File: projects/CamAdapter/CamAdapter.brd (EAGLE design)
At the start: 25.4 x 41.9 mm, 5 parts

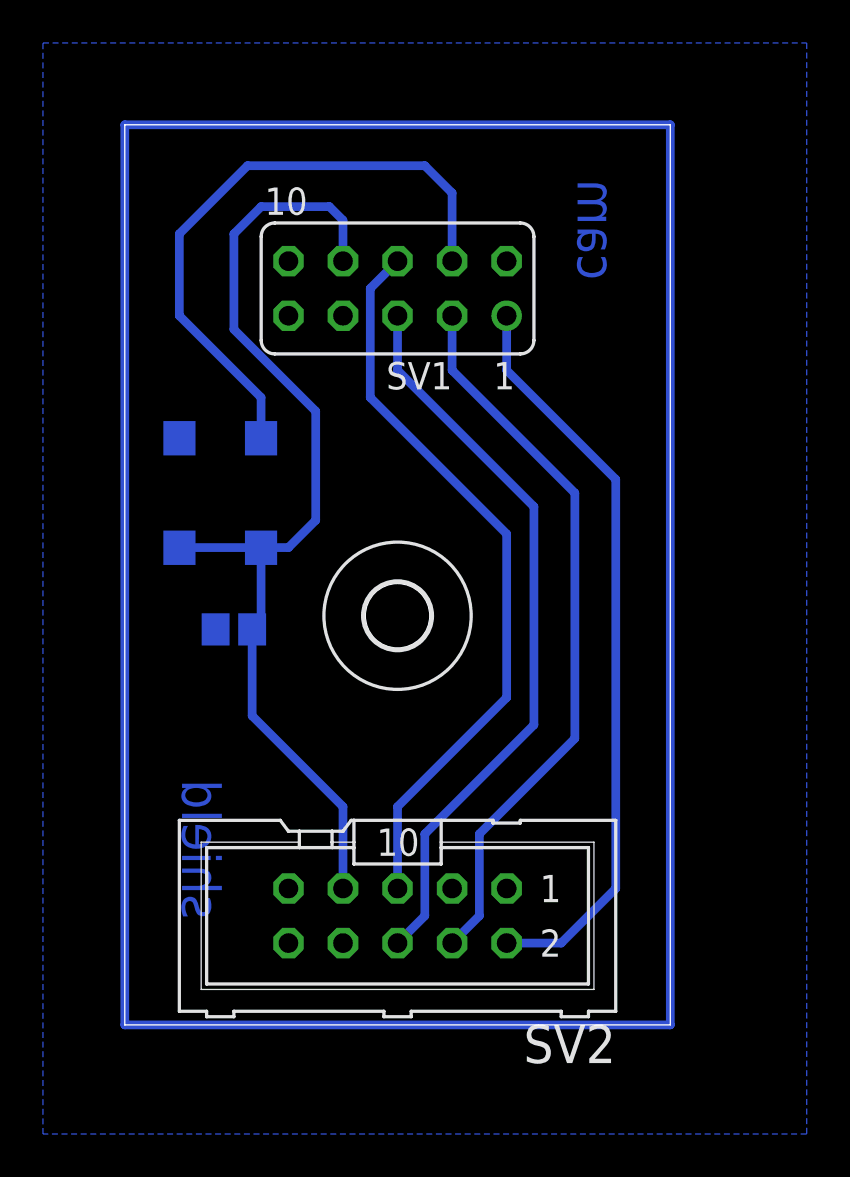
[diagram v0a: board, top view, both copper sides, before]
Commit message: pcb2gcode outline & drill test
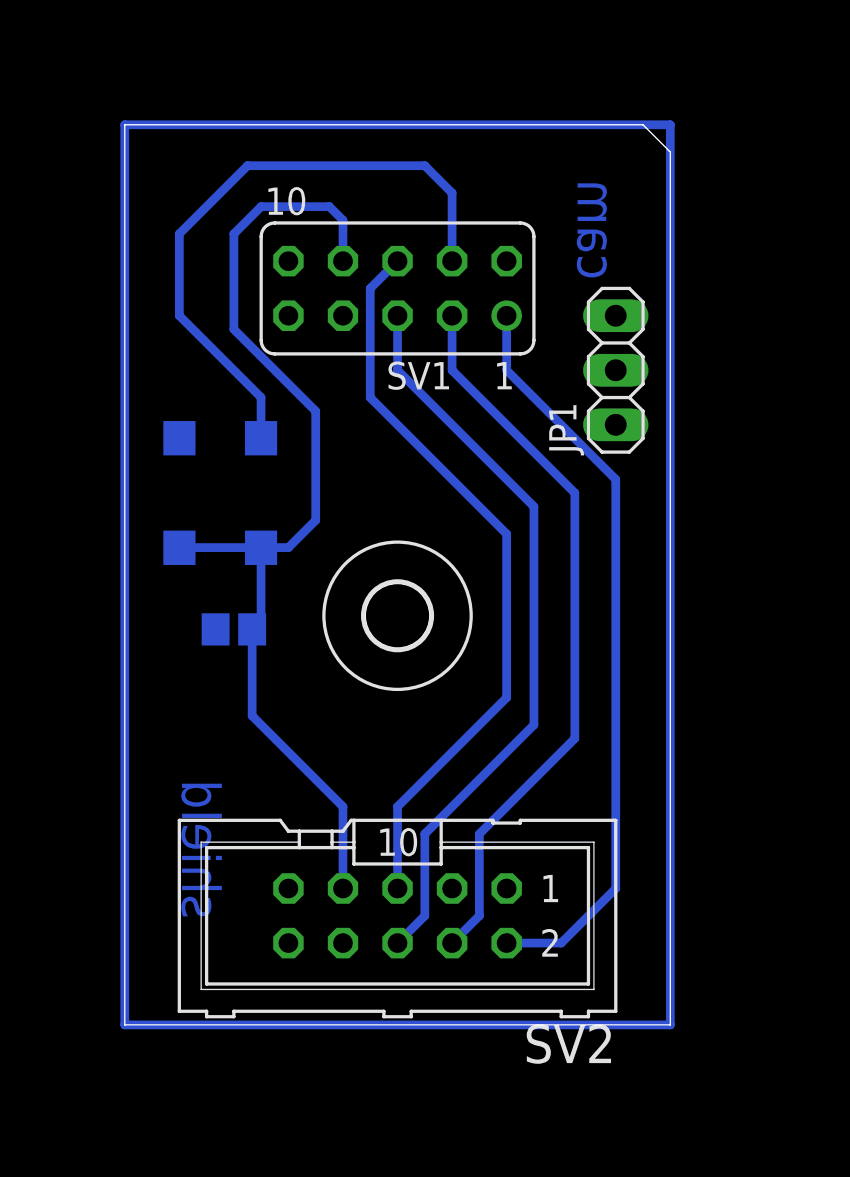
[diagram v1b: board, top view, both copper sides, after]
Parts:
- added JP1: (no value), pinhead:1X03
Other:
- outline, holes or cut-outs redrawn
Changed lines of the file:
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@@
 <board>
 <plain>
-<wire x1="0" y1="0" x2="25.4" y2="0" width="0" layer="20"/>
-<wire x1="25.4" y1="0" x2="25.4" y2="41.91" width="0" layer="20"/>
-<wire x1="25.4" y1="41.91" x2="0" y2="41.91" width="0" layer="20"/>
-<wire x1="0" y1="41.91" x2="0" y2="0" width="0" layer="20"/>
+<wire x1="0" y1="0" x2="25.4" y2="0" width="0.0254" layer="20"/>
+<wire x1="25.4" y1="0" x2="25.4" y2="40.64" width="0.0254" layer="20"/>
+<wire x1="25.4" y1="40.64" x2="24.13" y2="41.91" width="0.0254" layer="20"/>
+<wire x1="24.13" y1="41.91" x2="0" y2="41.91" width="0.0254" layer="20"/>
+<wire x1="0" y1="41.91" x2="0" y2="0" width="0.0254" layer="20"/>
 <text x="22.86" y="39.37" size="1.778" layer="16" font="vector" ratio="15" rot="MR270">cam</text>
 <text x="4.445" y="11.43" size="1.778" layer="16" font="vector" ratio="15" rot="MR270">shield</text>
@@
 </element>
 <element name="C1" library="resistor" package="C0805" value="100n" x="5.08" y="18.415" rot="MR0"/>
+<element name="JP1" library="pinhead" package="1X03" value="" x="22.86" y="30.48" rot="R90"/>
 </elements>
 <signals>
@@
 <contactref element="SV2" pad="9"/>
 <polygon width="0.4064" layer="16" isolate="0.3048">
-<vertex x="-3.81" y="45.72"/>
-<vertex x="31.75" y="45.72"/>
-<vertex x="31.75" y="-5.08"/>
-<vertex x="-3.81" y="-5.08"/>
+<vertex x="0" y="41.91"/>
+<vertex x="25.4" y="41.91"/>
+<vertex x="25.4" y="0"/>
+<vertex x="0" y="0"/>
 </polygon>
 <contactref element="SV1" pad="2"/>
@@
 <contactref element="QG1" pad="2"/>
 <contactref element="C1" pad="2"/>
+<wire x1="17.78" y1="6.35" x2="10.16" y2="3.81" width="0" layer="19" extent="1-1"/>
 </signal>
 <signal name="VCC">
